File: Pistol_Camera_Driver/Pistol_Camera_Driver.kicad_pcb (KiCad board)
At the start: 2 copper layers, 87.2 x 46.1 mm, 100 parts, among them J1 Screw_Terminal_01x02, J11 Screw_Terminal_01x02, J12 Screw_Terminal_01x02, J13 I2C, J14 Screw_Terminal_01x02, J15 Screw_Terminal_01x02, J16 Screw_Terminal_01x02, J17 Screw_Terminal_01x02, J18 Screw_Terminal_01x02, J19 I2C, J2 Objective, J3 Screw_Terminal_01x02, J4 Screw_Terminal_01x02, J5 Screw_Terminal_01x02, J6 Joystick, J7 Screw_Terminal_01x02, J8 Screw_Terminal_01x02, J9 Screw_Terminal_01x02, U1 XL1509-3.3, U12 MT3608, U2 XL1509-5.0, U4 DRV8834PWP, U5 DRV8834PWP

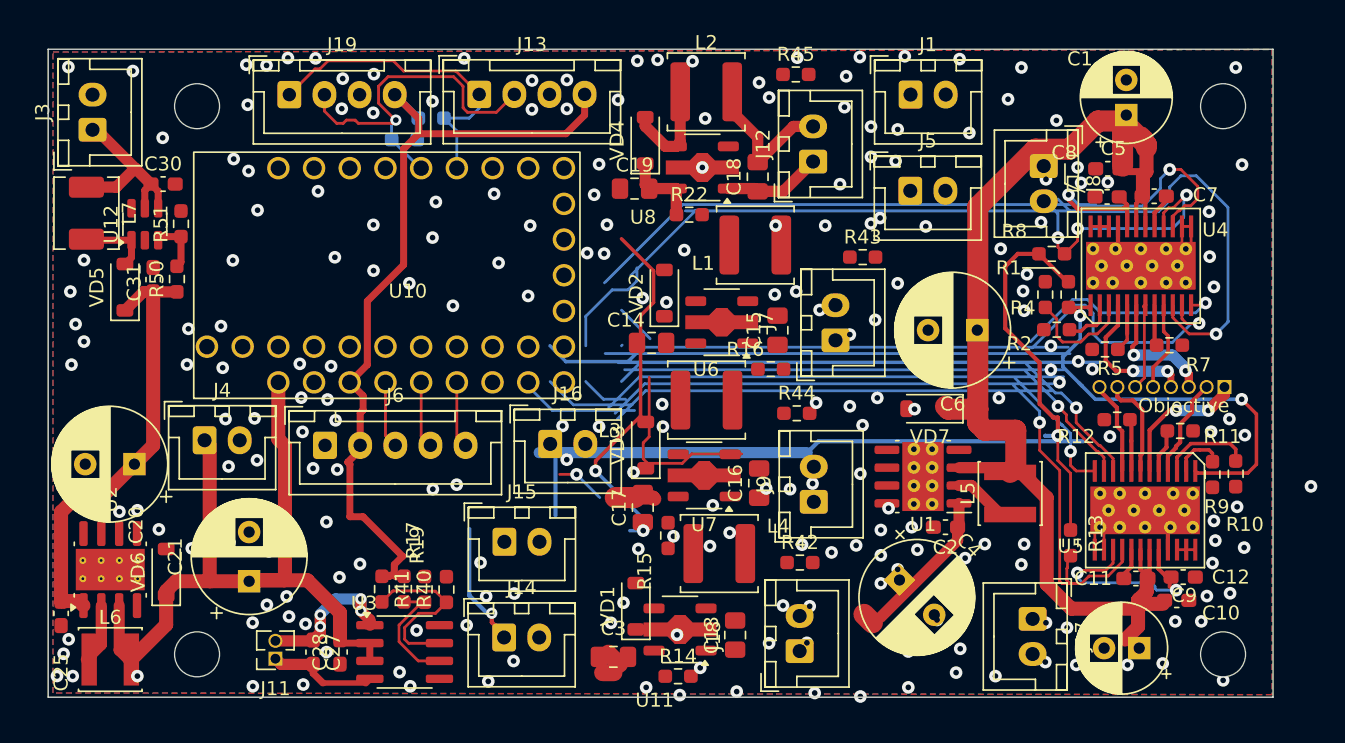
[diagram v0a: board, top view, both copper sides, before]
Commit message: v0.6 actual state
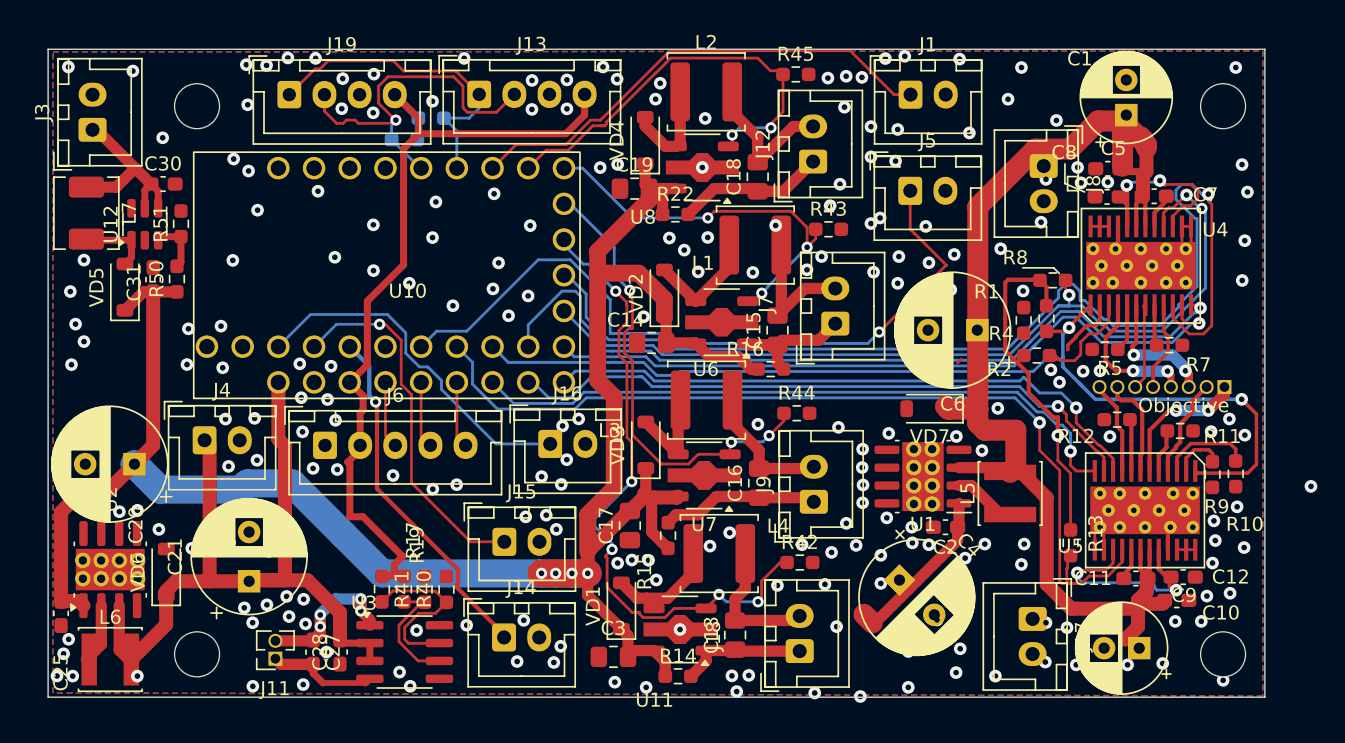
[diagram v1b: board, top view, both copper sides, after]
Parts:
- moved R43 3.14 mm to (85.6, 44.4)
- moved R4 2.39 mm to (99.5, 50.9)
- moved R2 2.32 mm to (100.4, 53.4)
- moved R1 2.31 mm to (101.1, 50.8)
- moved R8 1.89 mm to (101.5, 48.0)
- moved C17 1.58 mm to (71.4, 65.5)
- moved J7 1.19 mm to (86.1, 51.1)
- moved VD1 1.03 mm to (70.8, 71.2)
- moved R22 0.99 mm to (74.7, 43.4)
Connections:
- R42 pad 1: PWM_WHITE -> PWM_IR
- R45 pad 1: PWM_IR -> PWM_WHITE
- U11 pad 3: PWM_WHITE -> PWM_IR
- U8 pad 3: PWM_IR -> PWM_WHITE
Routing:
- net VPP: track 64.7 -> 147.8 mm, vias 1 -> 4
- net Net-(J7-Pin_1): track 64.0 -> 8.81 mm
- net K1: track 3.54 -> 52.9 mm
- net PWM_IR: track 0.00 -> 46.3 mm, vias 0 -> 5
- net Strobe Input: track 0.00 -> 34.5 mm
- net STEP1: track 18.1 -> 51.7 mm
- net DIR1: track 18.3 -> 50.9 mm
- net PWM_WHITE: track 0.00 -> 30.3 mm, vias 0 -> 2
- net Net-(J9-Pin_2): track 39.0 -> 9.60 mm
- net PWM_RED: track 0.00 -> 28.2 mm, vias 0 -> 3
- net K4: track 0.00 -> 26.3 mm, vias 0 -> 1
- net K5: track 0.00 -> 25.8 mm
- net PWM_UV: track 13.4 -> 33.4 mm, vias 0 -> 3
- net K3: track 8.64 -> 25.1 mm
- net Net-(J9-Pin_1): track 0.00 -> 11.3 mm
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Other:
- board size 87.2 x 46.1 mm -> 86.6 x 46.1 mm
